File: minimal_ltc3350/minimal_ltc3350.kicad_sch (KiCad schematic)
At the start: 85 parts, among them Q1 20.0 V, Q2 20.0 V, Q3 20 V, Q4 20 V, Q5 20.0 V, Q6 8 V, Q7 8 V, Q8 8 V, Q9 8 V, U1 LTC3350EUHF-PBF

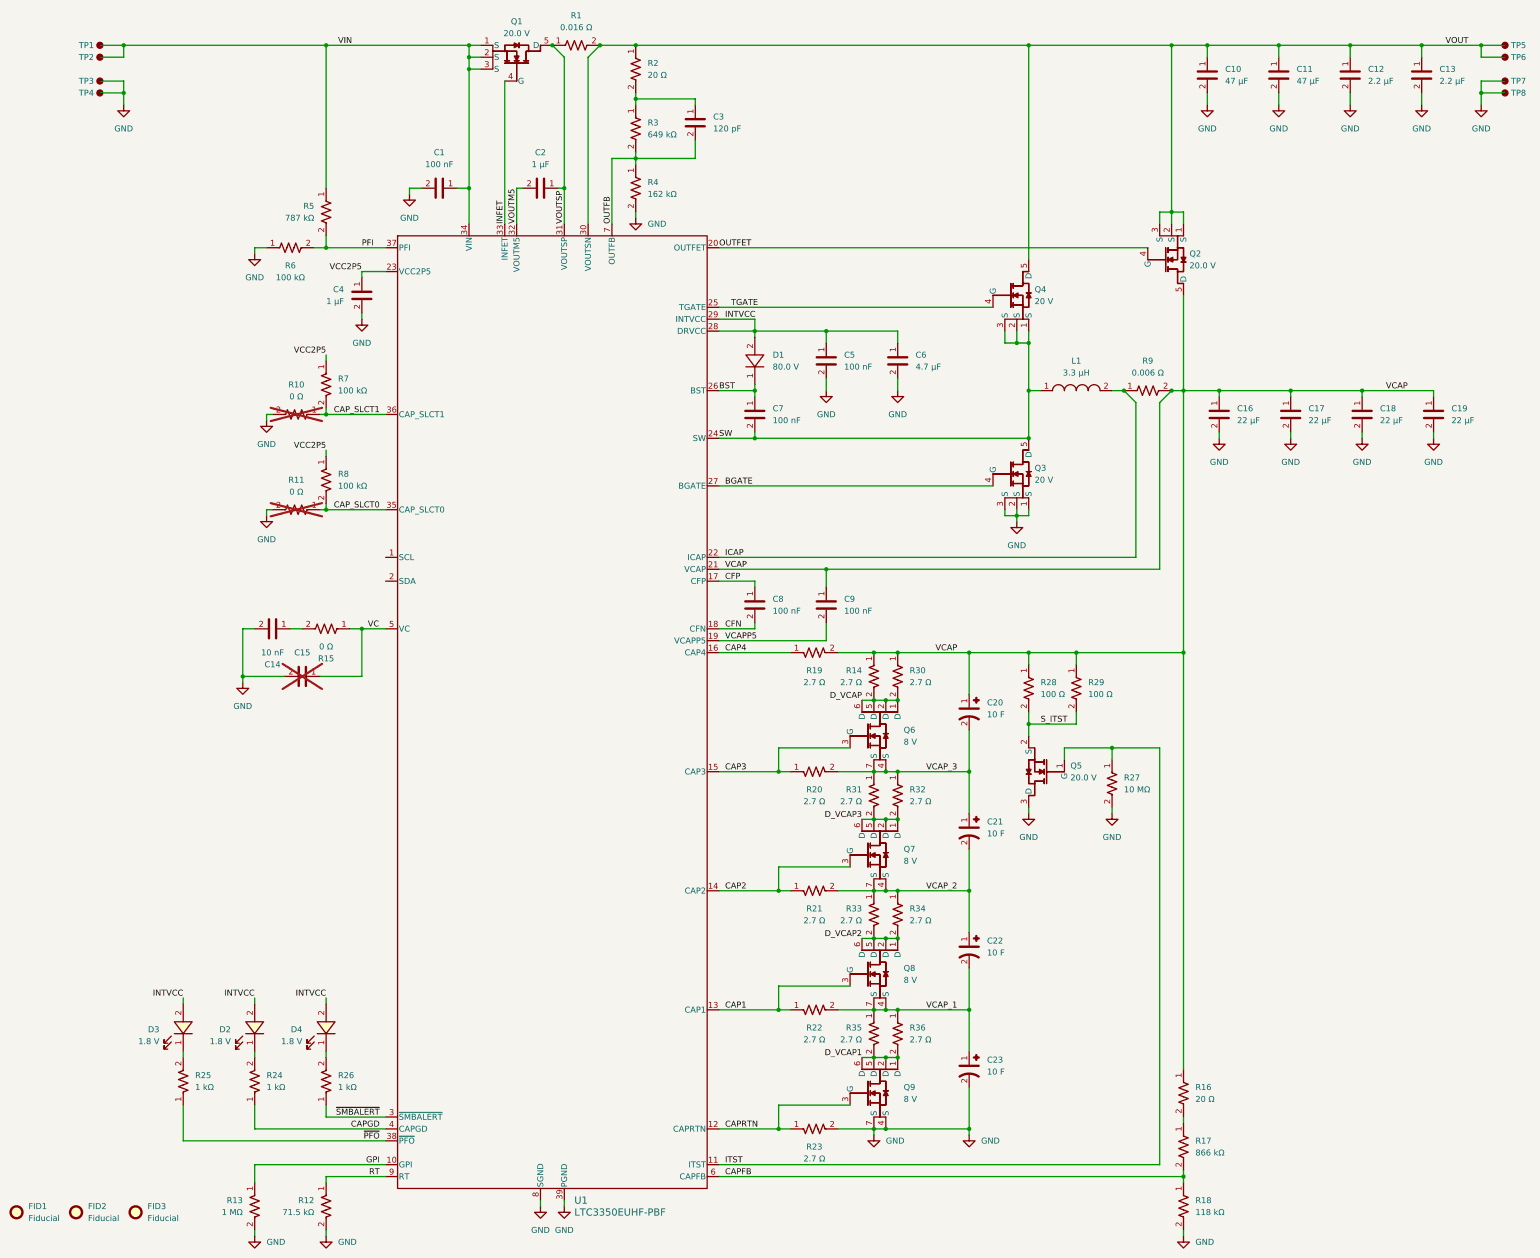
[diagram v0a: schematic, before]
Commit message: backup
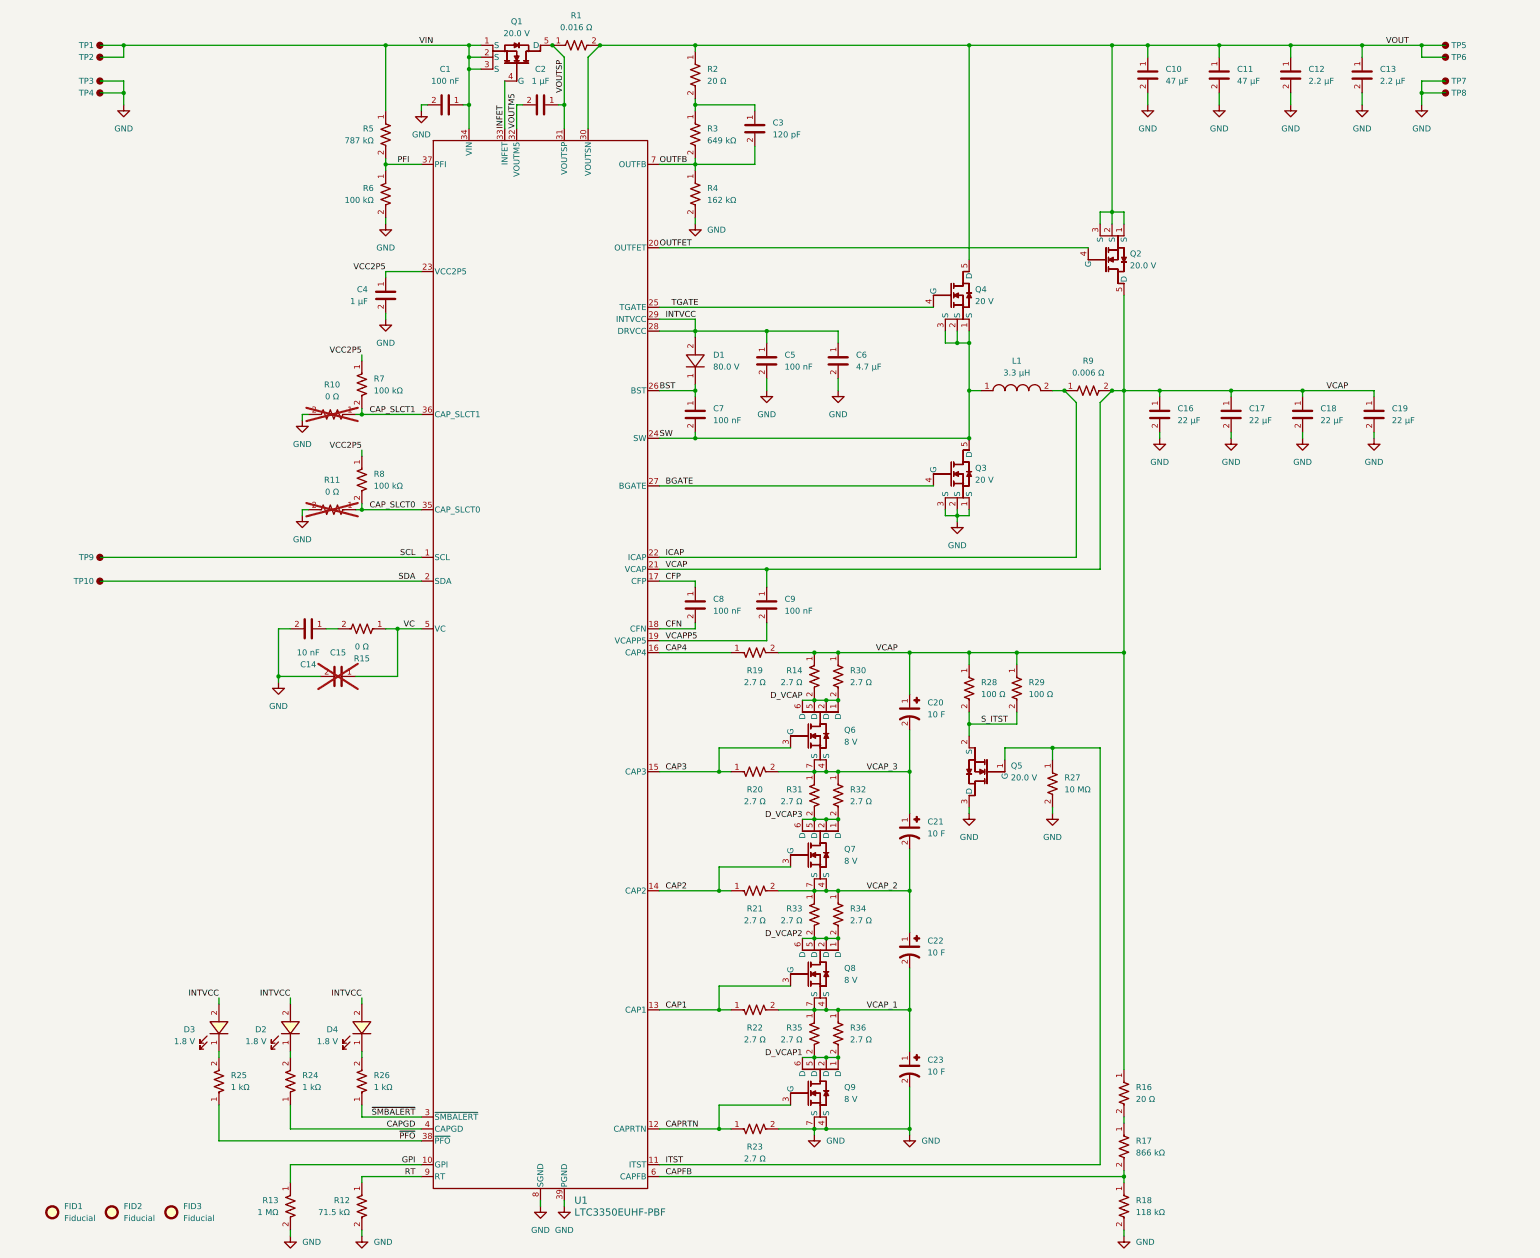
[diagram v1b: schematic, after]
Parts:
- added TP10, TP9: TestPoint, test_point_footprints:TestPoint_THTPad_Castelated, symbol UNITED_TEST_POINTS:TestPoint_Castelated_v2
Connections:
- net GND: now also R6.2; no longer R6.1
- net PFI: now also R6.1; no longer R6.2
- net SCL: now reaches U1.1 (SCL)
- net SCL: now also TP9.1
- net SDA: now reaches U1.2 (SDA)
- net SDA: now also TP10.1
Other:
- moved on the sheet: C1, C10, C11, C12, C13, C14, C15, C16, C17, C18, C19, C2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
